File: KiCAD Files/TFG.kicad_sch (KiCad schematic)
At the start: 43 parts, among them J1 Screw_Terminal_01x03, J2 Screw_Terminal_01x03, J3 Screw_Terminal_01x03, J4 Screw_Terminal_01x02, J5 Screw_Terminal_01x02, Q1 2N3906, Q2 2N3906, Q3 2N3906, Q4 2N3904, Q5 2N3904, Q6 2N3904, U1 L298HN, U2 ARDUINO_MKR_ZERO, U3 L7805

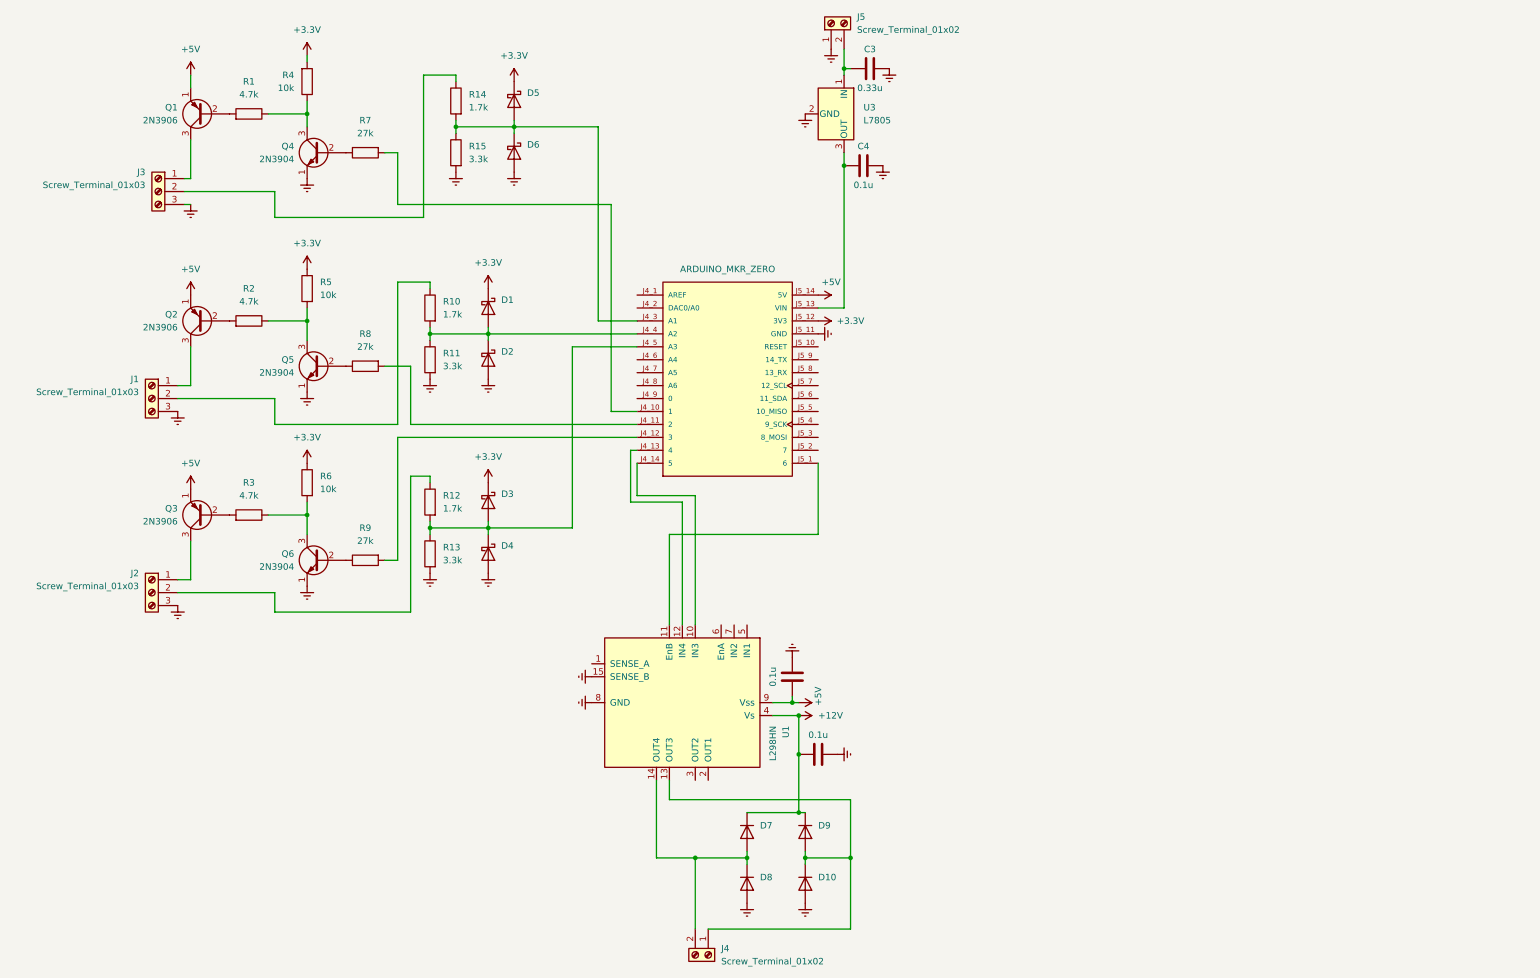
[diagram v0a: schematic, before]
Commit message: prettier sch
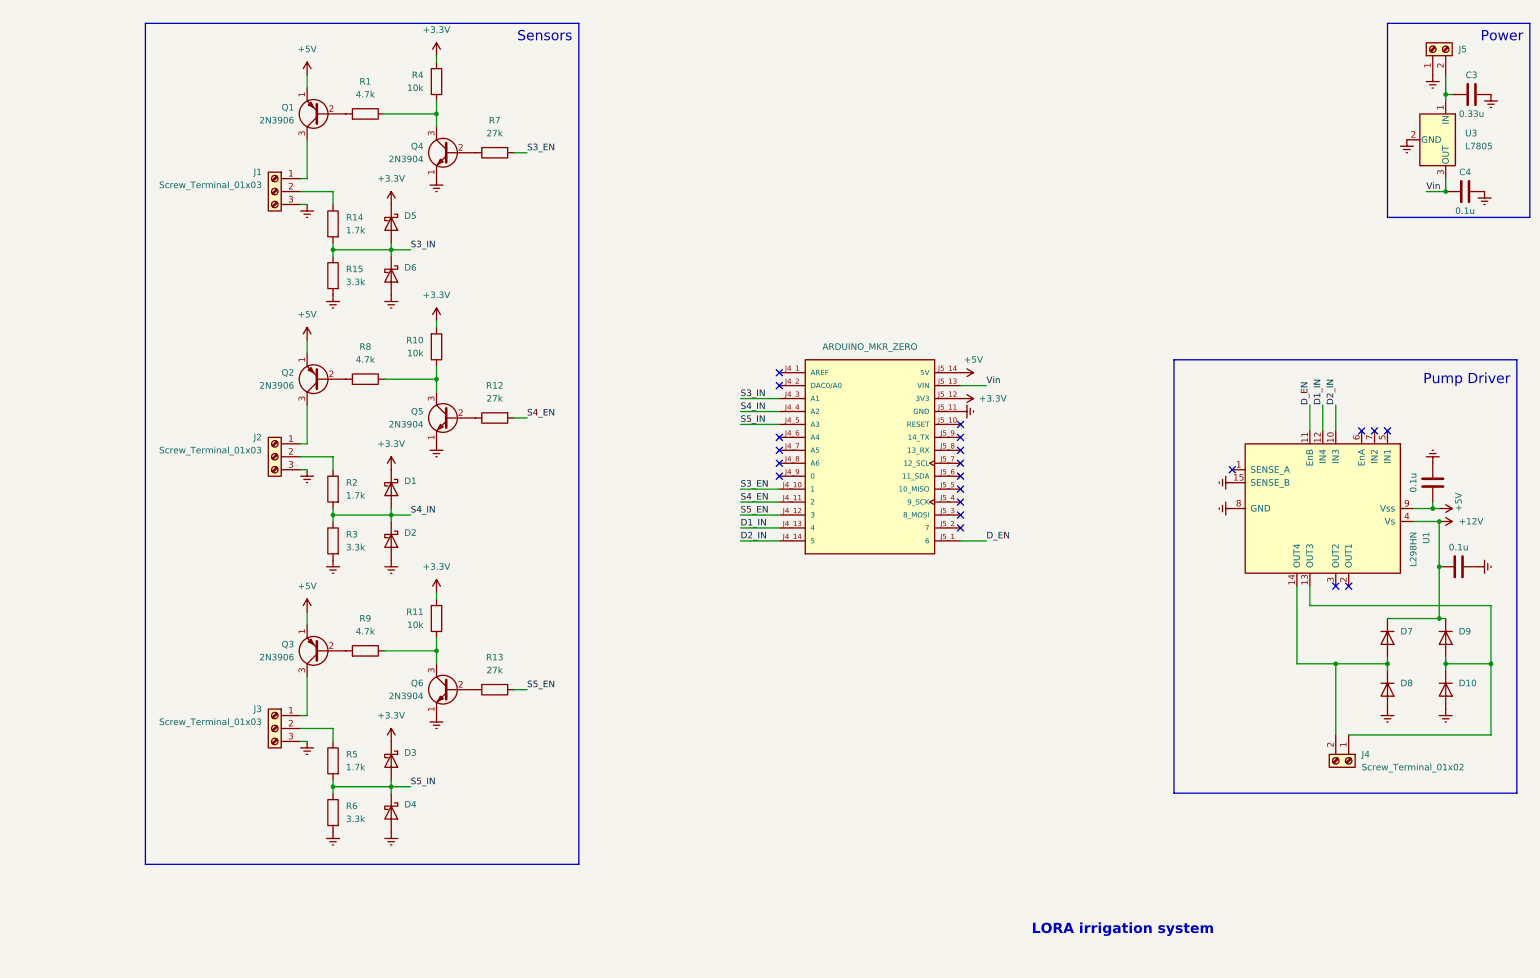
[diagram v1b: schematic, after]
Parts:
- removed J1: Screw_Terminal_01x03, TerminalBlock_Phoenix:TerminalBlock_Phoenix_MKDS-1,5-3_1x03_P5.00mm_Horizontal, symbol Connector:Screw_Terminal_01x03
- added J3: Screw_Terminal_01x03, TerminalBlock_Phoenix:TerminalBlock_Phoenix_MKDS-1,5-3_1x03_P5.00mm_Horizontal, symbol Connector:Screw_Terminal_01x03
- R10: value 1.7k -> 10k
- R11: value 3.3k -> 10k
- R12: value 1.7k -> 27k
- R13: value 3.3k -> 27k
- R2: value 4.7k -> 1.7k
- R3: value 4.7k -> 3.3k
- R5: value 10k -> 1.7k
- R6: value 10k -> 3.3k
- R8, R9: value 27k -> 4.7k
- renumbered J3 to J1
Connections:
- net +3V3: now also R10.2, R11.2; no longer R5.1, R6.1
- net Earth: now also R3.2, R6.2, J3.3 (Pin_3); no longer R11.2, R13.2
- net S5_IN: now reaches D3.2 (A), D4.1 (K), U2.J4_5 (A3)
- net S5_IN: now also R5.2, R6.1; no longer R12.2, R13.1
- net S4_IN: now reaches D1.2 (A), D2.1 (K), U2.J4_4 (A2)
- net S4_IN: now also R2.2, R3.1; no longer R10.2, R11.1
- net Vin: now reaches C4.1, U2.J5_13 (VIN), U3.3 (OUT)
- net at Q5.2 (B): now also R12.1; no longer R8.1
- net at Q6.2 (B): now also R13.1; no longer R9.1
- net at R9.2: now also Q3.2 (B); no longer U2.J4_12 (3)
- net D2_IN: now reaches U1.10 (IN3), U2.J4_14 (5)
- net D_EN: now reaches U1.11 (EnB), U2.J5_1 (6)
- net D1_IN: now reaches U1.12 (IN4), U2.J4_13 (4)
- net S3_EN: now reaches R7.2, U2.J4_10 (1)
- net at R8.2: now also Q2.2 (B); no longer U2.J4_11 (2)
- net S3_IN: now reaches D5.2 (A), D6.1 (K), R14.2, R15.1, U2.J4_3 (A1)
- net at J2.1 (Pin_1): now also Q2.3 (C); no longer Q3.3 (C)
- net at J2.2 (Pin_2): now also R2.1; no longer R12.1
- net at R10.1: now also Q5.3 (C), R8.1
- new net: Q6.3 (C), R11.1, R9.1
- new net: J3.2 (Pin_2), R5.1
- new net: J3.1 (Pin_1), Q3.3 (C)
- new net S4_EN: R12.2, U2.J4_11 (2)
- new net S5_EN: R13.2, U2.J4_12 (3)
- no-connect marks 0 -> 21
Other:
- note added: "LORA irrigation system"
- note added: "Power"
- note added: "Pump Driver"
- note added: "Sensors"
- moved on the sheet: C3, C4, D10, D5, D6, D7, D8, D9, J1, J4, J5, Q1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
